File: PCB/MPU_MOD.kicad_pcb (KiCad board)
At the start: 6 copper layers, 43.5 x 90 mm, 293 parts, among them J1 SJ-43504-SMT-TR, J2 2-1734248-0, J3 USB4510-03-1-A_REVA, J4 Conn_02x20_Odd_Even, J501 MEM2090-00-145-00-A_REVA, J701 FTSH-107-01-L-DV-K-A, J901 73412-0110, U201 STC3115IQT, U203 STPMIC1APQR, U3 BQ24298RTWR, U301 STM32MP157FABx, U401 MT41K256M16TW-107_P, U502 HSP051-4M10, U503 HSP051-4M10, U701 HSP051-4M10, U702 HSP051-4M10, U801 FUSB302BMPX, U802 HSP051-4M10, U901 LBEE5PK2AE-771, Y601 NX2012SA-32.768K, Y701 ECS-2520MVQ-240

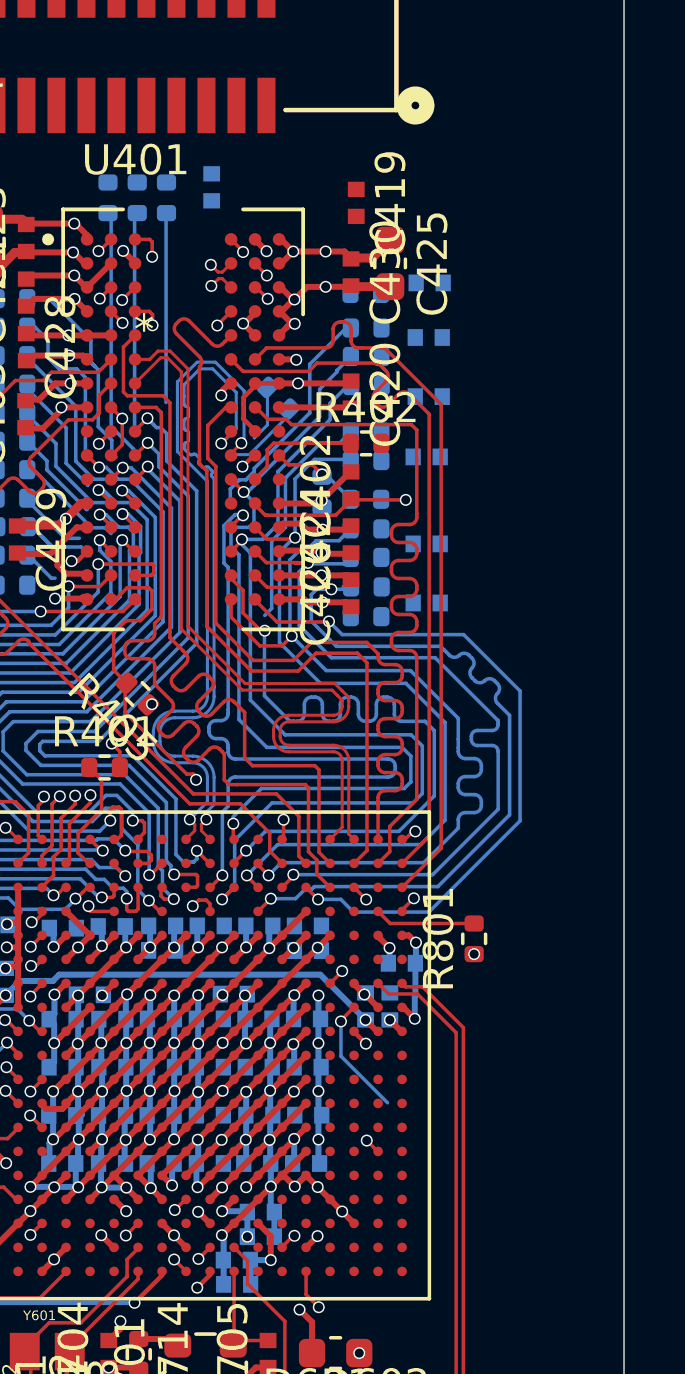
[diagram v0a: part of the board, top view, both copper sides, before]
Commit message: PCB_UPDATE
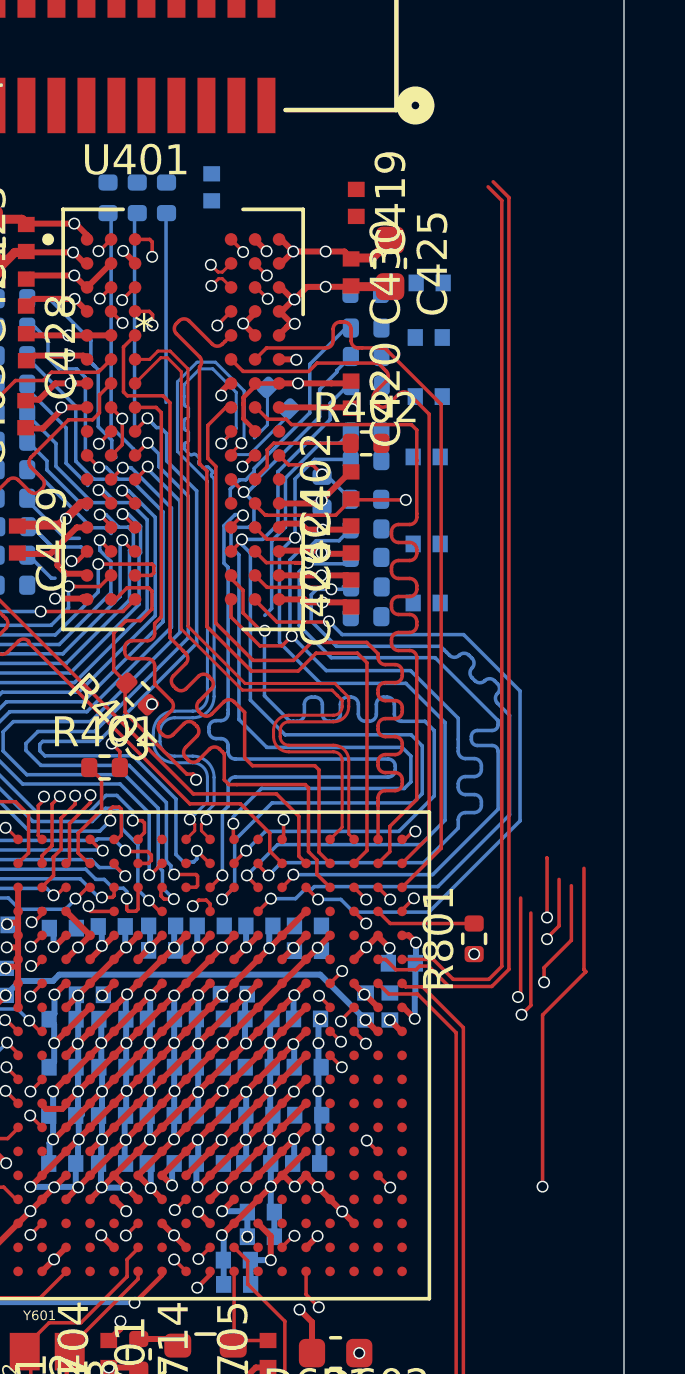
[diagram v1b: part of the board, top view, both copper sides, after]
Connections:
- U301 pad T10: unconnected-(U301D-PE7-PadT10) -> UART7_RX_STM
- U301 pad T11: unconnected-(U301D-PE8-PadT11) -> UART7_TX_STM
- U301 pad T12: unconnected-(U301C-PB6-PadT12) -> FDCAN2_TX
- U301 pad U16: unconnected-(U301C-PA12-PadU16) -> SYS_I2C6_SDA
- U301 pad V14: unconnected-(U301F-USB_DP1-PadV14) -> USB_M_D+
- U301 pad V17: unconnected-(U301C-PA11-PadV17) -> SYS_I2C6_SCL
- U301 pad V5: unconnected-(U301C-PB12-PadV5) -> FDCAN2_RX
- U301 pad W14: unconnected-(U301F-USB_DM1-PadW14) -> USB_M_D-
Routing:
- net USB_M_D+: track 0.00 -> 31.5 mm
- net USB_M_D-: track 0.00 -> 30.0 mm
- net FDCAN2_RX: track 0.00 -> 16.9 mm, vias 0 -> 2
- net FDCAN2_TX: track 0.00 -> 12.1 mm, vias 0 -> 2
- net UART7_RX_STM: track 0.00 -> 10.8 mm, vias 0 -> 2
- net UART7_TX_STM: track 0.00 -> 10.7 mm, vias 0 -> 2
- net SYS_I2C6_SDA: track 0.00 -> 8.97 mm, vias 0 -> 2
- net SYS_I2C6_SCL: track 0.00 -> 8.04 mm, vias 0 -> 2
- net SYS_I2C4_SCL: track 41.3 -> 43.8 mm
- net GND: track 191.8 -> 192.2 mm, vias 186 -> 187
